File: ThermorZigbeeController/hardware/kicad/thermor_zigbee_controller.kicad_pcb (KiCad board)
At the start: 2 copper layers, 80 x 60 mm, 6 parts, among them J1 PIR_SENSOR, U1 ESP32-C6-WROOM-1, U2 HT1621, U3 PC817

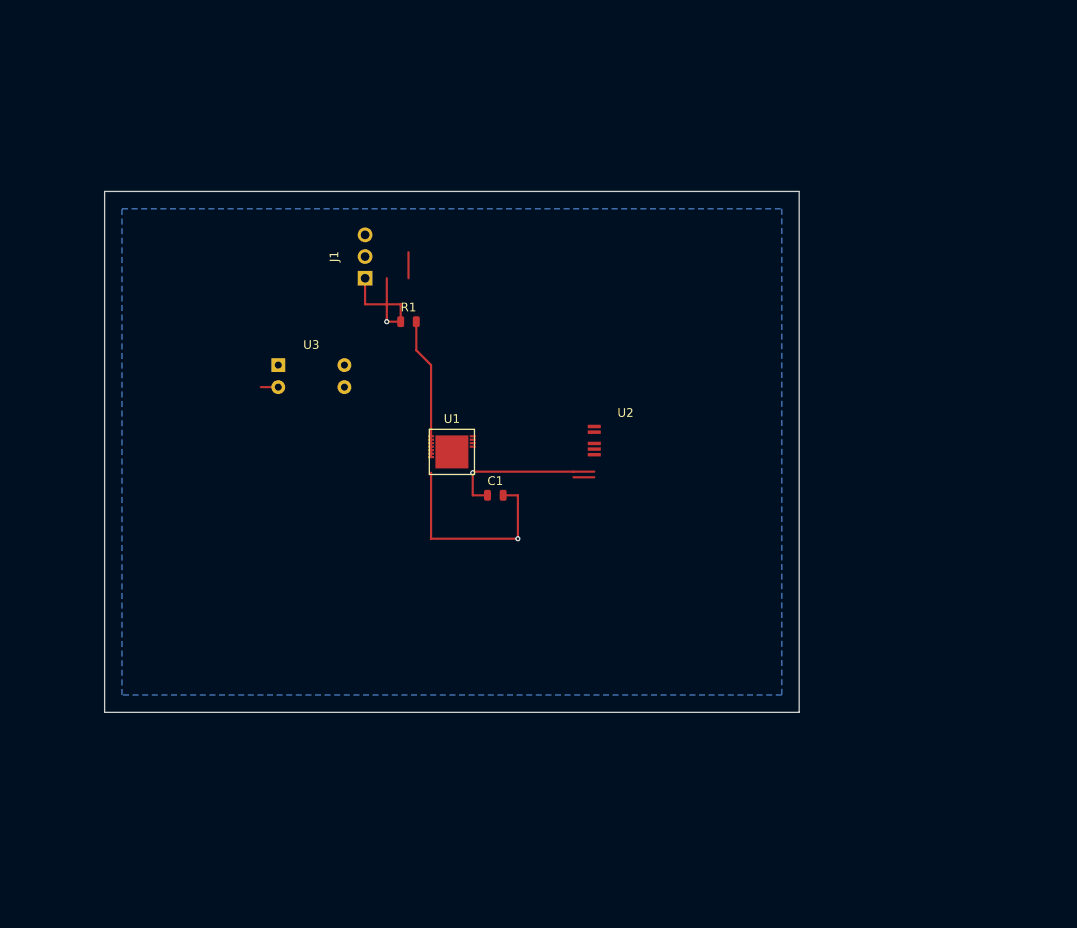
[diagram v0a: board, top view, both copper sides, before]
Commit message: Update
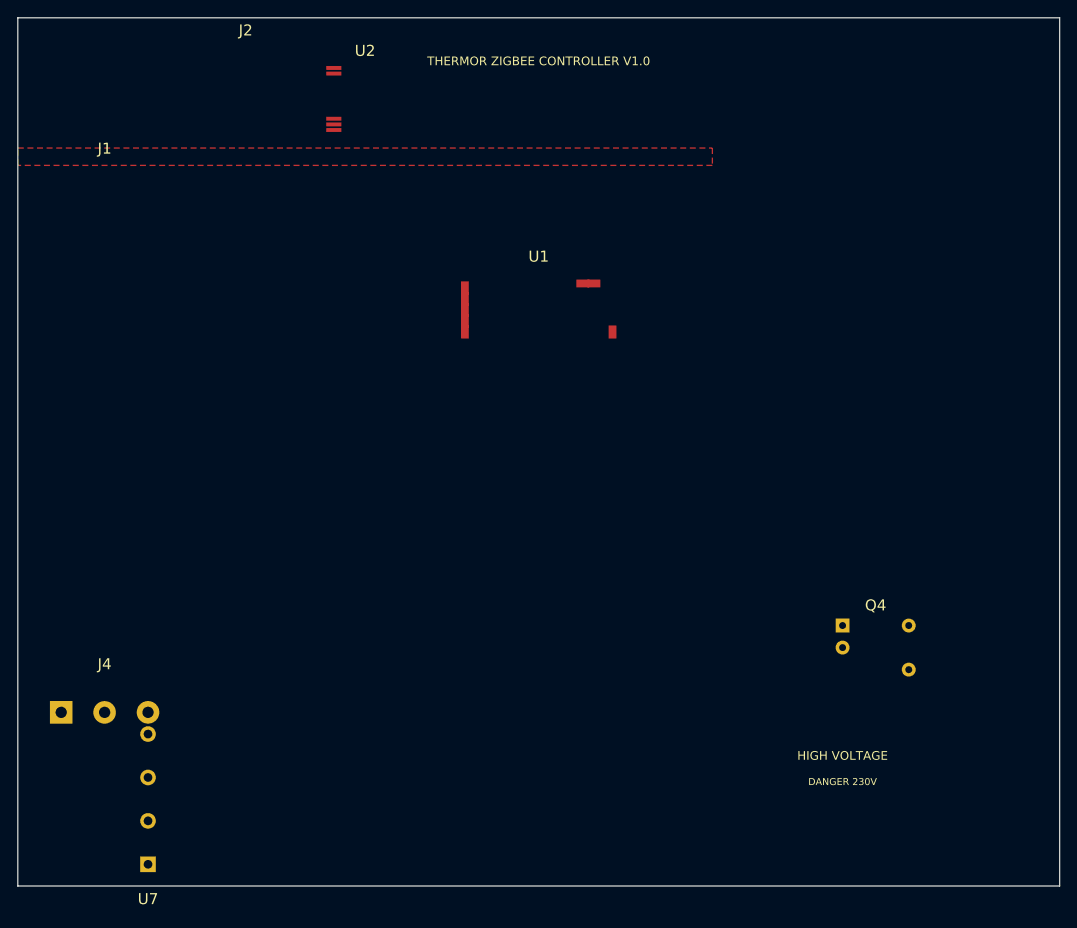
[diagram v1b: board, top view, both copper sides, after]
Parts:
- removed C1: 100nF, Capacitor_SMD:C_0805_2012Metric
- removed R1: 10k, Resistor_SMD:R_0805_2012Metric
- removed U3: PC817, Package_DIP:DIP-4_W7.62mm
- added J2: LCD_Conn, Connector_JST:JST_XH_B6B-XH-A_1x06_P2.50mm_Vertical, F.Cu at (120.0, 85.0)
- added J4: AC_Input, TerminalBlock_Phoenix:TerminalBlock_Phoenix_MKDS-1,5-3_1x03_P5.00mm_Horizontal, F.Cu at (105.0, 160.0)
- added Q4: MOC3021, Package_DIP:DIP-6_W7.62mm, F.Cu at (195.0, 150.0)
- added U7: HLK-PM03, Converter_ACDC:Converter_ACDC_HiLink_HLK-PMxx, F.Cu at (115.0, 170.0)
- J1: value PIR_SENSOR -> USB-C; footprint Connector_JST:JST_XH_B3B-XH-A_1x03_P2.50mm_Vertical -> Connector_USB:USB_C_Receptacle_USB2.0
- U1: footprint Package_DFN_QFN:QFN-40-1EP_5x5mm_P0.4mm_EP3.8x3.8mm -> RF_Module:ESP32-C6-WROOM-1
- U2: footprint Package_SO:SSOP-20_5.3x7.2mm_P0.65mm -> Package_SO:SSOP-28_5.3x10.2mm_P0.65mm
- moved U2 50.0 mm to (140.0, 90.0)
- moved J1 31.6 mm to (110.0, 100.0), turned to 0 degrees
- moved U1 14.1 mm to (160.0, 120.0)
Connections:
- U1 pad 1: GND -> +3V3
- U1 pad 2: +3V3 -> (no net)
- U1 pad 3: +3V3 -> LCD_CS
- U1 pad 4: /TRIAC1 -> LCD_WR
- U1 pad 5: /TRIAC2 -> LCD_DATA
- U2 pad 1: GND -> +3V3
- U2 pad 2: +3V3 -> GND
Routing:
- net GND: track 31.7 -> 0.00 mm, vias 1 -> 0
- net +3V3: track 27.4 -> 0.00 mm, vias 1 -> 0
- net /PIR_OUT: track 22.9 -> 0.00 mm, vias 1 -> 0
- added copper zone on F.Cu, net HV_ISOLATION
- removed copper zone on B.Cu, net GND
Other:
- board size 80 x 60 mm -> 120 x 100 mm
- board text added: "DANGER 230V"
- board text added: "HIGH VOLTAGE"
- board text added: "THERMOR ZIGBEE CONTROLLER V1.0"
